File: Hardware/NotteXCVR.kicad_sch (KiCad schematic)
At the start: 0 parts

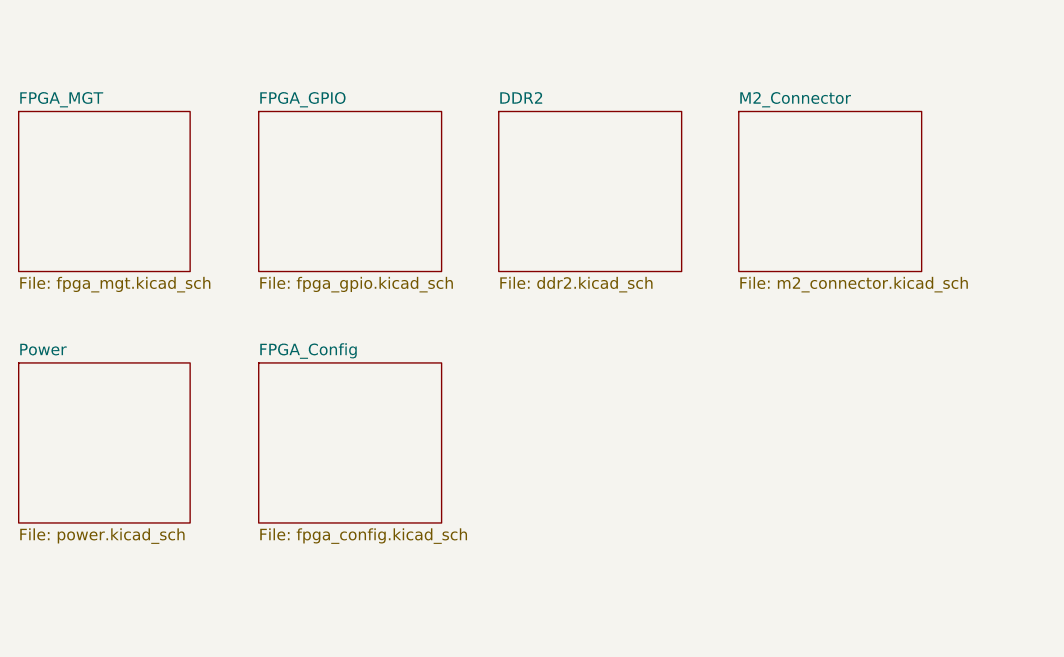
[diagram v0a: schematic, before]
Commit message: CSG325?
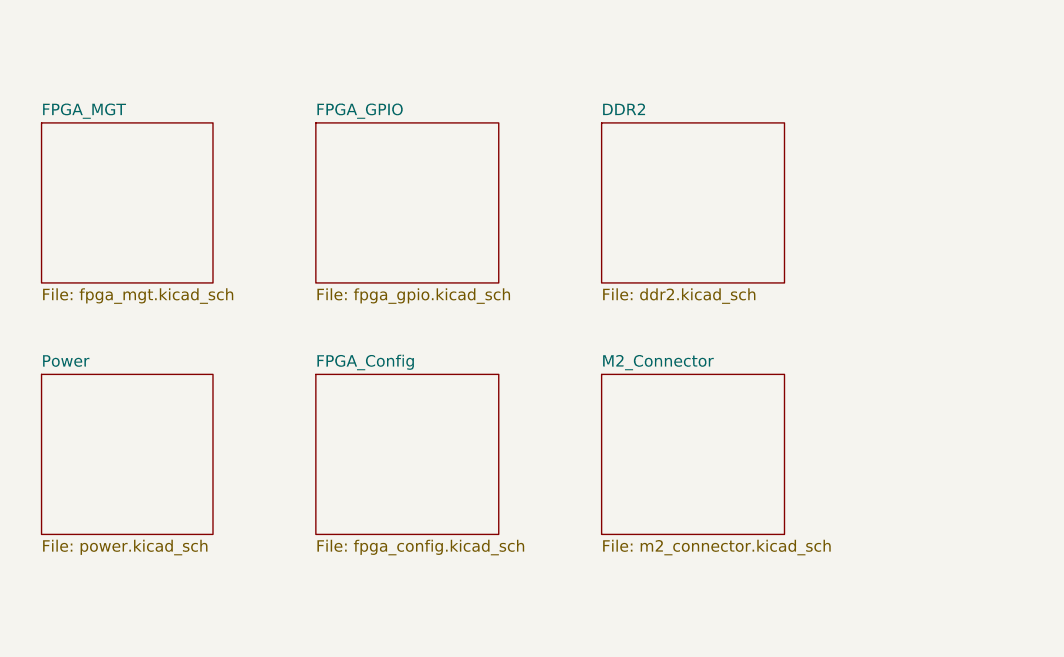
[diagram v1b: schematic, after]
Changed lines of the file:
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@@
 	(generator "eeschema")
 	(generator_version "10.0")
-	(paper "A4")
-	(sheet
-		(at 85.09 71.12)
+	(paper "B")
+	(sheet
+		(at 96.52 72.39)
 		(size 20.32 17.78)
 		(exclude_from_sim no)
@@
 		)
 		(property "Sheetname" "DDR2"
-			(at 85.09 70.4084 0)
+			(at 96.52 71.6784 0)
 			(show_name no)
 			(do_not_autoplace no)
@@
 		)
 		(property "Sheetfile" "ddr2.kicad_sch"
-			(at 85.09 89.4846 0)
+			(at 96.52 90.7546 0)
 			(show_name no)
 			(do_not_autoplace no)
@@
 	)
 	(sheet
-		(at 31.75 71.12)
+		(at 34.29 72.39)
 		(size 19.05 17.78)
 		(exclude_from_sim no)
@@
 		)
 		(property "Sheetname" "FPGA_MGT"
-			(at 31.75 70.4084 0)
+			(at 34.29 71.6784 0)
 			(show_name no)
 			(do_not_autoplace no)
@@
 		)
 		(property "Sheetfile" "fpga_mgt.kicad_sch"
-			(at 31.75 89.4846 0)
+			(at 34.29 90.7546 0)
 			(show_name no)
 			(do_not_autoplace no)
@@
 	)
 	(sheet
-		(at 58.42 71.12)
+		(at 64.77 72.39)
 		(size 20.32 17.78)
 		(exclude_from_sim no)
@@
 		)
 		(property "Sheetname" "FPGA_GPIO"
-			(at 58.42 70.4084 0)
+			(at 64.77 71.6784 0)
 			(show_name no)
 			(do_not_autoplace no)
@@
 		)
 		(property "Sheetfile" "fpga_gpio.kicad_sch"
-			(at 58.42 89.4846 0)
+			(at 64.77 90.7546 0)
 			(show_name no)
 			(do_not_autoplace no)
@@
 	)
 	(sheet
-		(at 111.76 71.12)
+		(at 96.52 100.33)
 		(size 20.32 17.78)
 		(exclude_from_sim no)
@@
 		)
 		(property "Sheetname" "M2_Connector"
-			(at 111.76 70.4084 0)
+			(at 96.52 99.6184 0)
 			(show_name no)
 			(do_not_autoplace no)
@@
 		)
 		(property "Sheetfile" "m2_connector.kicad_sch"
-			(at 111.76 89.4846 0)
+			(at 96.52 118.6946 0)
 			(show_name no)
 			(do_not_autoplace no)
@@
 	)
 	(sheet
-		(at 58.42 99.06)
+		(at 64.77 100.33)
 		(size 20.32 17.78)
 		(exclude_from_sim no)
@@
 		)
 		(property "Sheetname" "FPGA_Config"
-			(at 58.42 98.3484 0)
+			(at 64.77 99.6184 0)
 			(show_name no)
 			(do_not_autoplace no)
@@
 		)
 		(property "Sheetfile" "fpga_config.kicad_sch"
-			(at 58.42 117.4246 0)
+			(at 64.77 118.6946 0)
 			(show_name no)
 			(do_not_autoplace no)
@@
 	)
 	(sheet
-		(at 31.75 99.06)
+		(at 34.29 100.33)
 		(size 19.05 17.78)
 		(exclude_from_sim no)
@@
 		)
 		(property "Sheetname" "Power"
-			(at 31.75 98.3484 0)
+			(at 34.29 99.6184 0)
 			(show_name no)
 			(do_not_autoplace no)
@@
 		)
 		(property "Sheetfile" "power.kicad_sch"
-			(at 31.75 117.4246 0)
-			(show_name no)
-			(do_not_autoplace no)
+			(at 34.29 118.6946 0)
+			(show_name no)
+			(do_not_autoplace no)

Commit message: PCIe
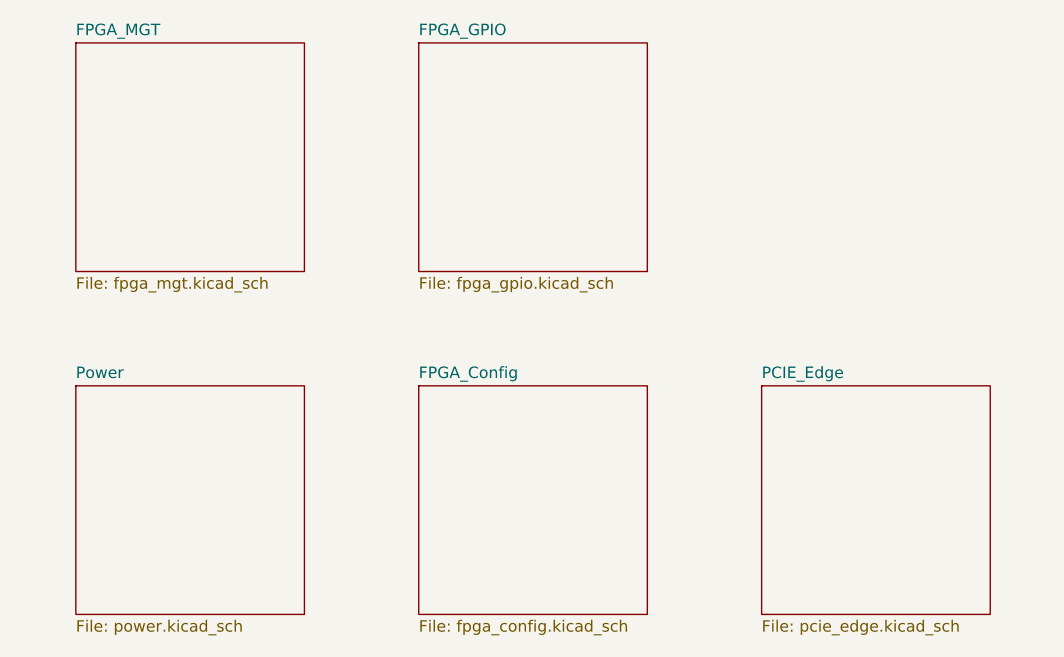
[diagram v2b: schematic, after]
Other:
- removed sheet DDR2
- removed sheet M2_Connector
- added sheet PCIE_Edge (pcie_edge.kicad_sch)
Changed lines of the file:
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@@
 	(paper "B")
 	(sheet
-		(at 96.52 72.39)
-		(size 20.32 17.78)
-		(exclude_from_sim no)
-		(in_bom yes)
-		(on_board yes)
-		(dnp no)
-		(fields_autoplaced yes)
-		(stroke
-			(width 0.1524)
-			(type solid)
-		)
-		(fill
-			(color 0 0 0 0)
-		)
-		(property "Sheetname" "DDR2"
-			(at 96.52 71.6784 0)
-			(show_name no)
-			(do_not_autoplace no)
-			(effects
-				(font
-					(size 1.27 1.27)
-				)
-				(justify left bottom)
-			)
-		)
-		(property "Sheetfile" "ddr2.kicad_sch"
-			(at 96.52 90.7546 0)
+		(at 38.1 63.5)
+		(size 25.4 25.4)
+		(exclude_from_sim no)
+		(in_bom yes)
+		(on_board yes)
+		(dnp no)
+		(fields_autoplaced yes)
+		(stroke
+			(width 0.1524)
+			(type solid)
+		)
+		(fill
+			(color 0 0 0 0)
+		)
+		(property "Sheetname" "FPGA_MGT"
+			(at 38.1 62.7884 0)
+			(show_name no)
+			(do_not_autoplace no)
+			(effects
+				(font
+					(size 1.27 1.27)
+				)
+				(justify left bottom)
+			)
+		)
+		(property "Sheetfile" "fpga_mgt.kicad_sch"
+			(at 38.1 89.4846 0)
+			(show_name no)
+			(do_not_autoplace no)
+			(effects
+				(font
+					(size 1.27 1.27)
+				)
+				(justify left top)
+			)
+		)
+		(instances
+			(project "NotteXCVR"
+				(path "/66cb547b-932d-4f9e-941e-9414e44abcf1"
+					(page "2")
+				)
+			)
+		)
+	)
+	(sheet
+		(at 76.2 63.5)
+		(size 25.4 25.4)
+		(exclude_from_sim no)
+		(in_bom yes)
+		(on_board yes)
+		(dnp no)
+		(fields_autoplaced yes)
+		(stroke
+			(width 0.1524)
+			(type solid)
+		)
+		(fill
+			(color 0 0 0 0)
+		)
+		(property "Sheetname" "FPGA_GPIO"
+			(at 76.2 62.7884 0)
+			(show_name no)
+			(do_not_autoplace no)
+			(effects
+				(font
+					(size 1.27 1.27)
+				)
+				(justify left bottom)
+			)
+		)
+		(property "Sheetfile" "fpga_gpio.kicad_sch"
+			(at 76.2 89.4846 0)
+			(show_name no)
+			(do_not_autoplace no)
+			(effects
+				(font
+					(size 1.27 1.27)
+				)
+				(justify left top)
+			)
+		)
+		(instances
+			(project "NotteXCVR"
+				(path "/66cb547b-932d-4f9e-941e-9414e44abcf1"
+					(page "3")
+				)
+			)
+		)
+	)
+	(sheet
+		(at 76.2 101.6)
+		(size 25.4 25.4)
+		(exclude_from_sim no)
+		(in_bom yes)
+		(on_board yes)
+		(dnp no)
+		(fields_autoplaced yes)
+		(stroke
+			(width 0.1524)
+			(type solid)
+		)
+		(fill
+			(color 0 0 0 0)
+		)
+		(property "Sheetname" "FPGA_Config"
+			(at 76.2 100.8884 0)
+			(show_name no)
+			(do_not_autoplace no)
+			(effects
+				(font
+					(size 1.27 1.27)
+				)
+				(justify left bottom)
+			)
+		)
+		(property "Sheetfile" "fpga_config.kicad_sch"
+			(at 76.2 127.5846 0)
+			(show_name no)
+			(do_not_autoplace no)
+			(effects
+				(font
+					(size 1.27 1.27)
+				)
+				(justify left top)
+			)
+		)
+		(instances
+			(project "NotteXCVR"
+				(path "/66cb547b-932d-4f9e-941e-9414e44abcf1"
+					(page "7")
+				)
+			)
+		)
+	)
+	(sheet
+		(at 38.1 101.6)
+		(size 25.4 25.4)
+		(exclude_from_sim no)
+		(in_bom yes)
+		(on_board yes)
+		(dnp no)
+		(fields_autoplaced yes)
+		(stroke
+			(width 0.1524)
+			(type solid)
+		)
+		(fill
+			(color 0 0 0 0)
+		)
+		(property "Sheetname" "Power"
+			(at 38.1 100.8884 0)
+			(show_name no)
+			(do_not_autoplace no)
+			(effects
+				(font
+					(size 1.27 1.27)
+				)
+				(justify left bottom)
+			)
+		)
+		(property "Sheetfile" "power.kicad_sch"
+			(at 38.1 127.5846 0)
+			(show_name no)
+			(do_not_autoplace no)
+			(effects
+				(font
+					(size 1.27 1.27)
+				)
+				(justify left top)
+			)
+		)
+		(instances
+			(project "NotteXCVR"
+				(path "/66cb547b-932d-4f9e-941e-9414e44abcf1"
+					(page "6")
+				)
+			)
+		)
+	)
+	(sheet
+		(at 114.3 101.6)
+		(size 25.4 25.4)
+		(exclude_from_sim no)
+		(in_bom yes)
+		(on_board yes)
+		(dnp no)
+		(fields_autoplaced yes)
+		(stroke
+			(width 0.1524)
+			(type solid)
+		)
+		(fill
+			(color 0 0 0 0)
+		)
+		(property "Sheetname" "PCIE_Edge"
+			(at 114.3 100.8884 0)
+			(show_name no)
+			(do_not_autoplace no)
+			(effects
+				(font
+					(size 1.27 1.27)
+				)
+				(justify left bottom)
+			)
+		)
+		(property "Sheetfile" "pcie_edge.kicad_sch"
+			(at 114.3 127.5846 0)
 			(show_name no)
 			(do_not_autoplace no)
@@
 				)
 			)
-		)
-	)
-	(sheet
-		(at 34.29 72.39)
-		(size 19.05 17.78)
-		(exclude_from_sim no)
-		(in_bom yes)
-		(on_board yes)
-		(dnp no)
-		(fields_autoplaced yes)
-		(stroke
-			(width 0.1524)
-			(type solid)
-		)
-		(fill
-			(color 0 0 0 0)
-		)
-		(property "Sheetname" "FPGA_MGT"
-			(at 34.29 71.6784 0)
-			(show_name no)
-			(do_not_autoplace no)
-			(effects
-				(font
-					(size 1.27 1.27)
-				)
-				(justify left bottom)
-			)
-		)
-		(property "Sheetfile" "fpga_mgt.kicad_sch"
-			(at 34.29 90.7546 0)
-			(show_name no)
-			(do_not_autoplace no)
-			(effects
-				(font
-					(size 1.27 1.27)
-				)
-				(justify left top)
-			)
-		)
-		(instances
-			(project "NotteXCVR"
-				(path "/66cb547b-932d-4f9e-941e-9414e44abcf1"
-					(page "2")
-				)
-			)
-		)
-	)
-	(sheet
-		(at 64.77 72.39)
-		(size 20.32 17.78)
-		(exclude_from_sim no)
-		(in_bom yes)
-		(on_board yes)
-		(dnp no)
-		(fields_autoplaced yes)
-		(stroke
-			(width 0.1524)
-			(type solid)
-		)
-		(fill
-			(color 0 0 0 0)
-		)
-		(property "Sheetname" "FPGA_GPIO"
-			(at 64.77 71.6784 0)
-			(show_name no)
-			(do_not_autoplace no)
-			(effects
-				(font
-					(size 1.27 1.27)
-				)
-				(justify left bottom)
-			)
-		)
-		(property "Sheetfile" "fpga_gpio.kicad_sch"
-			(at 64.77 90.7546 0)
-			(show_name no)
-			(do_not_autoplace no)
-			(effects
-				(font
-					(size 1.27 1.27)
-				)
-				(justify left top)
-			)
-		)
-		(instances
-			(project "NotteXCVR"
-				(path "/66cb547b-932d-4f9e-941e-9414e44abcf1"
-					(page "3")
-				)
-			)
-		)
-	)
-	(sheet
-		(at 96.52 100.33)
-		(size 20.32 17.78)
-		(exclude_from_sim no)
-		(in_bom yes)
-		(on_board yes)
-		(dnp no)
-		(fields_autoplaced yes)
-		(stroke
-			(width 0.1524)
-			(type solid)
-		)
-		(fill
-			(color 0 0 0 0)
-		)
-		(property "Sheetname" "M2_Connector"
-			(at 96.52 99.6184 0)
-			(show_name no)
-			(do_not_autoplace no)
-			(effects
-				(font
-					(size 1.27 1.27)
-				)
-				(justify left bottom)
-			)
-		)
-		(property "Sheetfile" "m2_connector.kicad_sch"
-			(at 96.52 118.6946 0)
-			(show_name no)
-			(do_not_autoplace no)
-			(effects
-				(font
-					(size 1.27 1.27)
-				)
-				(justify left top)
-			)
-		)
-		(instances
-			(project "NotteXCVR"
-				(path "/66cb547b-932d-4f9e-941e-9414e44abcf1"
-					(page "5")
-				)
-			)
-		)
-	)
-	(sheet
-		(at 64.77 100.33)
-		(size 20.32 17.78)
-		(exclude_from_sim no)
-		(in_bom yes)
-		(on_board yes)
-		(dnp no)
-		(fields_autoplaced yes)
-		(stroke
-			(width 0.1524)
-			(type solid)
-		)
-		(fill
-			(color 0 0 0 0)
-		)
-		(property "Sheetname" "FPGA_Config"
-			(at 64.77 99.6184 0)
-			(show_name no)
-			(do_not_autoplace no)
-			(effects
-				(font
-					(size 1.27 1.27)
-				)
-				(justify left bottom)
-			)
-		)
-		(property "Sheetfile" "fpga_config.kicad_sch"
-			(at 64.77 118.6946 0)
-			(show_name no)
-			(do_not_autoplace no)
-			(effects
-				(font
-					(size 1.27 1.27)
-				)
-				(justify left top)
-			)
-		)
-		(instances
-			(project "NotteXCVR"
-				(path "/66cb547b-932d-4f9e-941e-9414e44abcf1"
-					(page "7")
-				)
-			)
-		)
-	)
-	(sheet
-		(at 34.29 100.33)
-		(size 19.05 17.78)
-		(exclude_from_sim no)
-		(in_bom yes)
-		(on_board yes)
-		(dnp no)
-		(fields_autoplaced yes)
-		(stroke
-			(width 0.1524)
-			(type solid)
-		)
-		(fill
-			(color 0 0 0 0)
-		)
-		(property "Sheetname" "Power"
-			(at 34.29 99.6184 0)
-			(show_name no)
-			(do_not_autoplace no)
-			(effects
-				(font
-					(size 1.27 1.27)
-				)
-				(justify left bottom)
-			)
-		)
-		(property "Sheetfile" "power.kicad_sch"
-			(at 34.29 118.6946 0)
-			(show_name no)
-			(do_not_autoplace no)
-			(effects
-				(font
-					(size 1.27 1.27)
-				)
-				(justify left top)
-			)
-		)
-		(instances
-			(project "NotteXCVR"
-				(path "/66cb547b-932d-4f9e-941e-9414e44abcf1"
-					(page "6")
-				)
-			)
